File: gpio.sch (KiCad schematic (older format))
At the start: 3 parts, among them J1 DF40C-100DP-0.4V(51), J2 DF40C-100DP-0.4V(51), U1 LFE5U-85F-6BG381C

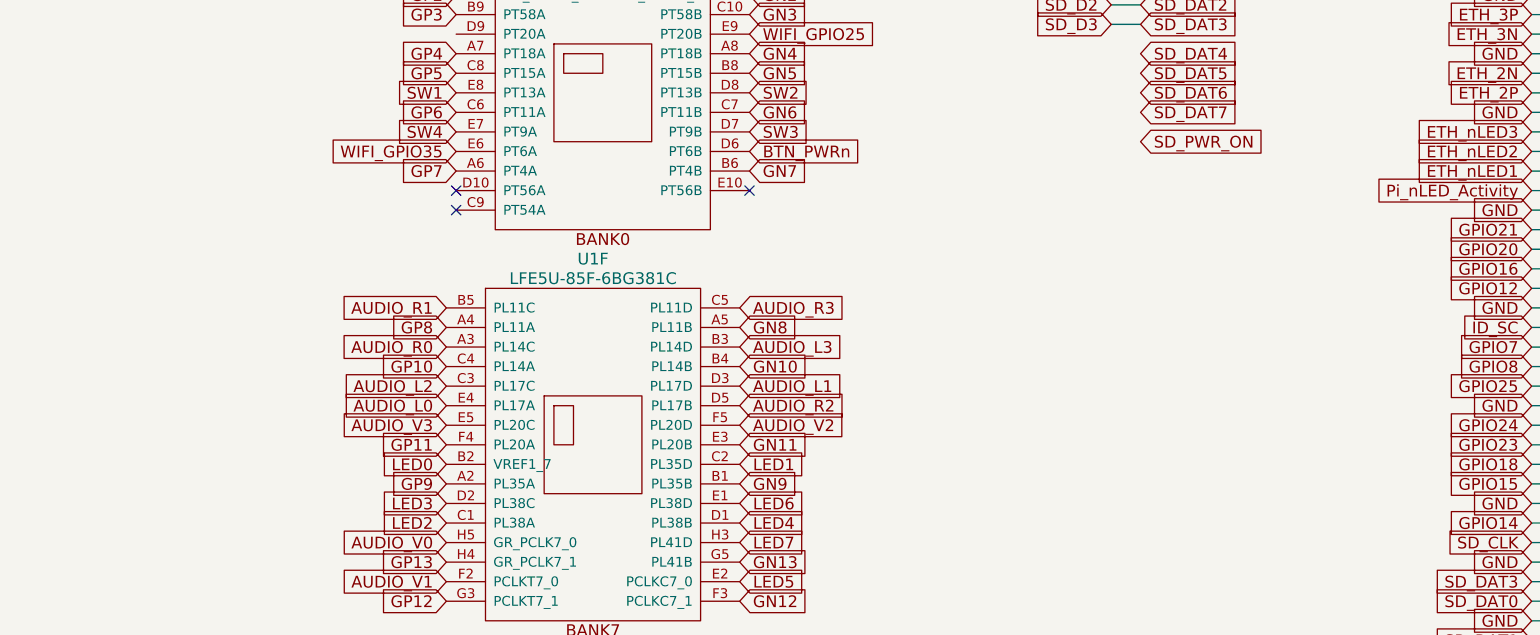
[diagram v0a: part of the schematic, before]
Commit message: SDRAM, JTAG routed - before logo delete
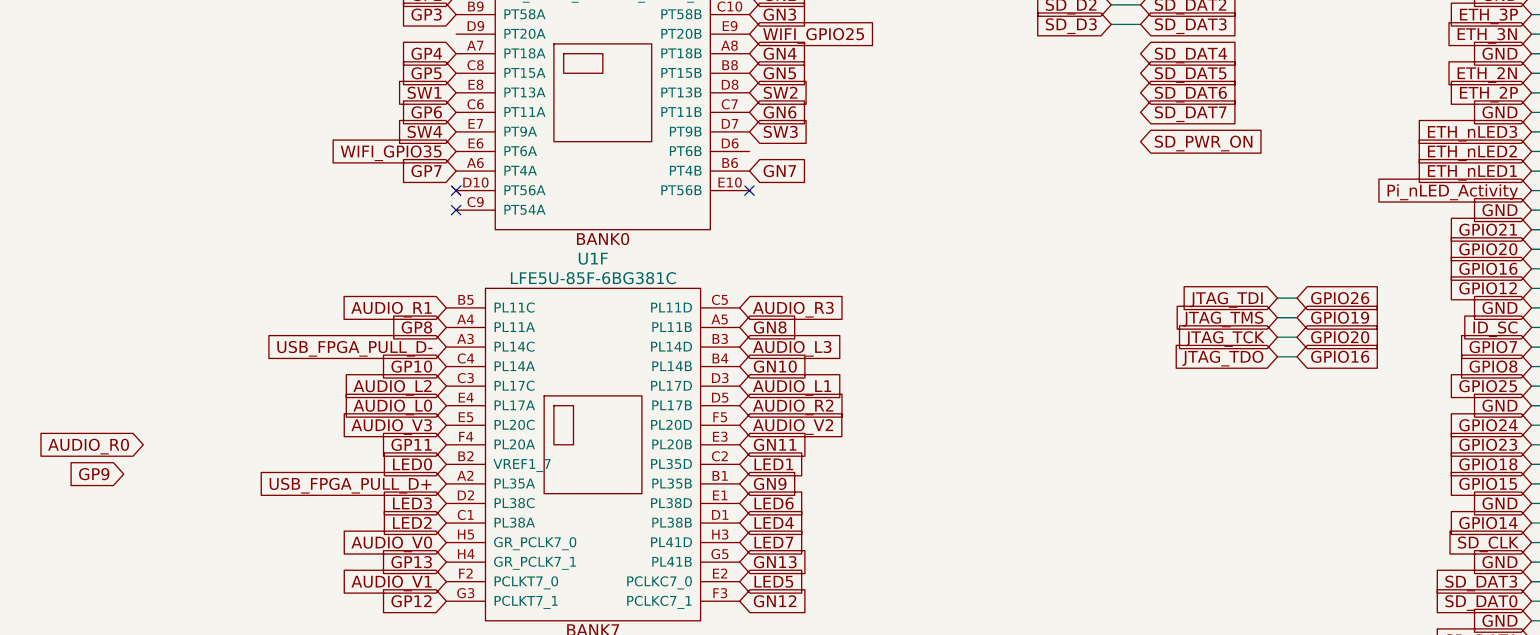
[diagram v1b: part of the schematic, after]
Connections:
- net AUDIO_R0: no longer U1.A3 (PL14C)
- net GP9: no longer U1.A2 (PL35A)
- net BTN_PWRn: no longer names the net of U1.D6 (PT6B)
- new net USB_FPGA_PULL_D+: U1.A2 (PL35A)
- new net USB_FPGA_PULL_D-: U1.A3 (PL14C)
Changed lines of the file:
@@
 Text GLabel 2550 3500 2    60   Input ~ 0
 GN9
-Text GLabel 1050 3500 0    60   Input ~ 0
+Text GLabel -600 3450 0    60   Input ~ 0
 GP9
 Text GLabel 2550 2900 2    60   Input ~ 0
@@
 Text GLabel 2550 2800 2    60   Input ~ 0
 AUDIO_L3
-Text GLabel 1050 2800 0    60   Input ~ 0
+Text GLabel -500 3300 0    60   Input ~ 0
 AUDIO_R0
 Text GLabel 1050 2600 0    60   Input ~ 0
@@
 Text Notes 950  7550 0    60   ~ 0
 GPIO route only A/B pairs as those are differential bidirectional\ndon't route C/D pairs to GPIO as those can be differential input only\nBANK0,1 are single-ended (non-differential)
-Text GLabel 2600 1800 2    60   Input ~ 0
-BTN_PWRn
 Text Notes 950  7200 0    60   ~ 0
 GP,GN 14-21 differential bidirectional connected to BANK2,3 on "ram" sheet\nGP,GN 22-27 single-ended connected to BANK1 on "gpdi" sheet
@@
 Wire Wire Line
 	4600 1150 4450 1150
+Text GLabel 1050 3500 0    60   Input ~ 0
+USB_FPGA_PULL_D+
+Text GLabel 1050 2800 0    60   Input ~ 0
+USB_FPGA_PULL_D-
+Text GLabel 5300 2550 0    60   Input ~ 0
+JTAG_TDI
+Text GLabel 5300 2650 0    60   Input ~ 0
+JTAG_TMS
+Text GLabel 5300 2750 0    60   Input ~ 0
+JTAG_TCK
+Text GLabel 5300 2850 0    60   Input ~ 0
+JTAG_TDO
+Text GLabel 5400 2550 2    60   Input ~ 0
+GPIO26
+Text GLabel 5400 2650 2    60   Input ~ 0
+GPIO19
+Text GLabel 5400 2850 2    60   Input ~ 0
+GPIO16
+Wire Wire Line
+	5300 2550 5400 2550
+Wire Wire Line
+	5400 2650 5300 2650
+Text GLabel 5400 2750 2    60   Input ~ 0
+GPIO20
+Wire Wire Line
+	5300 2750 5400 2750
+Wire Wire Line
+	5400 2850 5300 2850
 $EndSCHEMATC

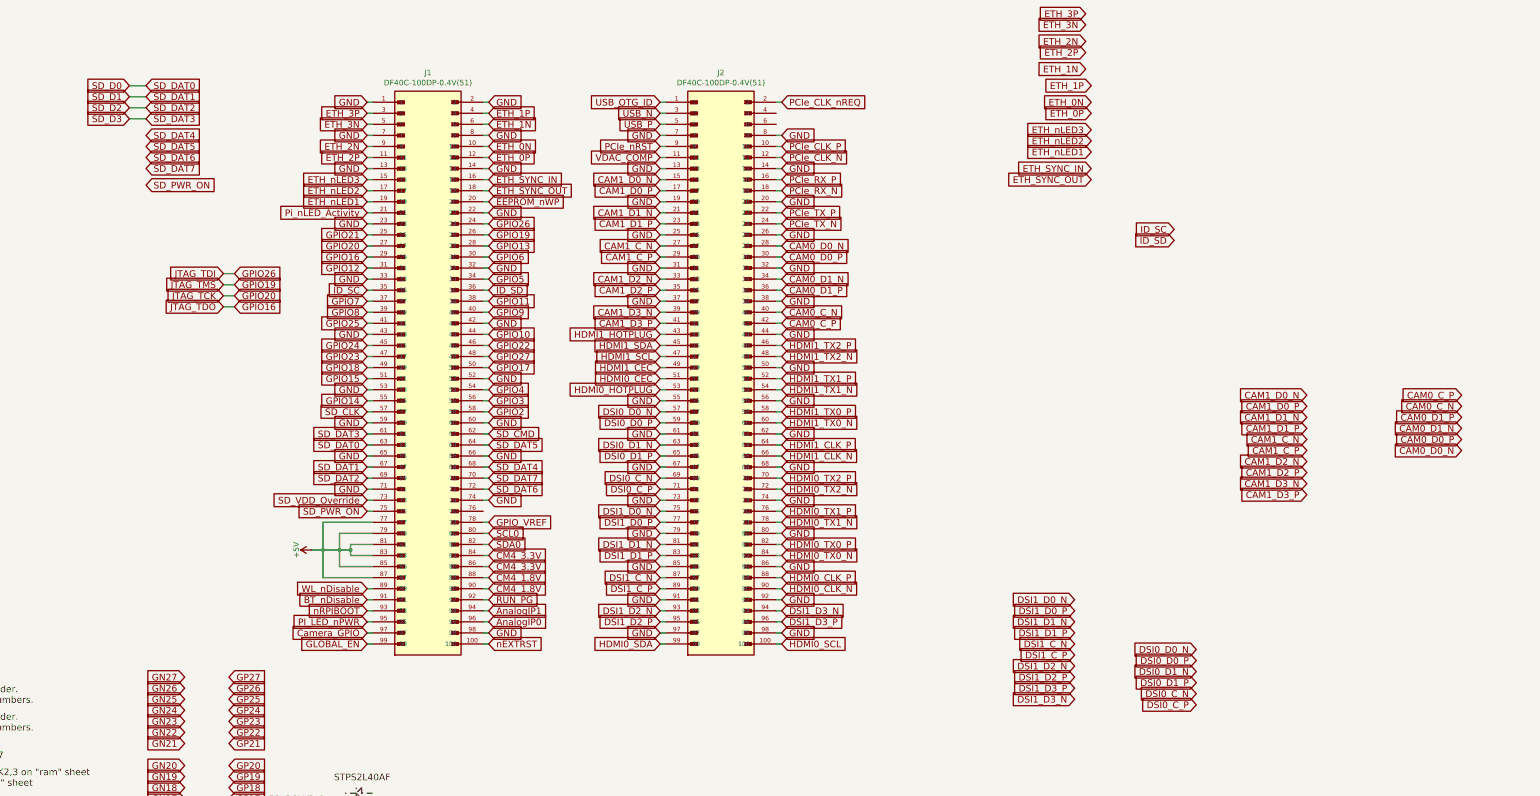
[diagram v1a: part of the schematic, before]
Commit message: Cleaning DRC errors
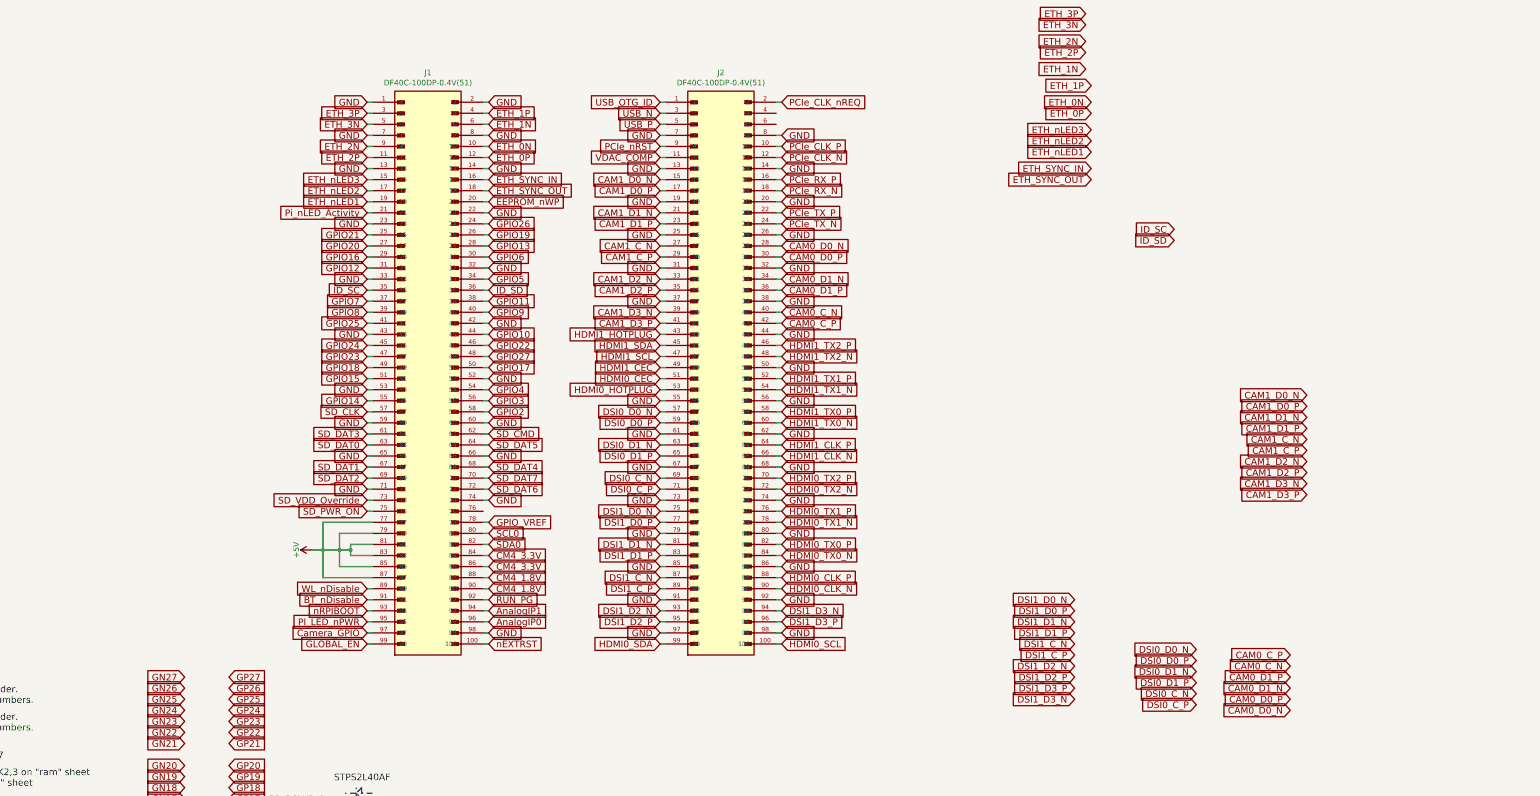
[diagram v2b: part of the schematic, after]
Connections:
- net SD_D0 renamed SD_DAT0
- net SD_D1 renamed SD_DAT1
- net SD_D2 renamed SD_DAT2
- net SD_D3 renamed SD_DAT3
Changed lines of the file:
@@
 Text GLabel 18150 2350 0    60   Input ~ 0
 GPIO21
-Text GLabel 16500 4150 0    60   Input ~ 0
+Text GLabel 14950 6500 0    60   Input ~ 0
 CAM0_D0_N
-Text GLabel 16500 4050 0    60   Input ~ 0
+Text GLabel 14950 6400 0    60   Input ~ 0
 CAM0_D0_P
-Text GLabel 16500 3950 0    60   Input ~ 0
+Text GLabel 14950 6300 0    60   Input ~ 0
 CAM0_D1_N
-Text GLabel 16500 3850 0    60   Input ~ 0
+Text GLabel 14950 6200 0    60   Input ~ 0
 CAM0_D1_P
-Text GLabel 16500 3750 0    60   Input ~ 0
+Text GLabel 14950 6100 0    60   Input ~ 0
 CAM0_C_N
-Text GLabel 16500 3650 0    60   Input ~ 0
+Text GLabel 14950 6000 0    60   Input ~ 0
 CAM0_C_P
 Text GLabel 15100 3650 0    60   Input ~ 0
@@
 Text GLabel 14100 5950 0    60   Input ~ 0
 DSI0_D0_N
-Text GLabel 4450 1050 0    60   Input ~ 0
-SD_D2
-Text GLabel 4450 1150 0    60   Input ~ 0
-SD_D3
-Text GLabel 4450 850  0    60   Input ~ 0
-SD_D0
-Text GLabel 4450 950  0    60   Input ~ 0
-SD_D1
-Text GLabel 4600 1050 2    60   Input ~ 0
-SD_DAT2
-Text GLabel 4600 950  2    60   Input ~ 0
-SD_DAT1
-Text GLabel 4600 1300 2    60   Input ~ 0
-SD_DAT4
-Text GLabel 4600 1400 2    60   Input ~ 0
-SD_DAT5
-Text GLabel 4600 1500 2    60   Input ~ 0
-SD_DAT6
-Text GLabel 4600 1600 2    60   Input ~ 0
-SD_DAT7
-Text GLabel 4600 1150 2    60   Input ~ 0
-SD_DAT3
-Text GLabel 4600 850  2    60   Input ~ 0
-SD_DAT0
-Text GLabel 4600 1750 2    60   Input ~ 0
-SD_PWR_ON
-Wire Wire Line
-	4450 850  4600 850
-Wire Wire Line
-	4600 950  4450 950
-Wire Wire Line
-	4450 1050 4600 1050
-Wire Wire Line
-	4600 1150 4450 1150
 Text GLabel 1050 3500 0    60   Input ~ 0
 USB_FPGA_PULL_D+
 Text GLabel 1050 2800 0    60   Input ~ 0
 USB_FPGA_PULL_D-
-Text GLabel 5300 2550 0    60   Input ~ 0
-JTAG_TDI
-Text GLabel 5300 2650 0    60   Input ~ 0
-JTAG_TMS
-Text GLabel 5300 2750 0    60   Input ~ 0
-JTAG_TCK
-Text GLabel 5300 2850 0    60   Input ~ 0
-JTAG_TDO
-Text GLabel 5400 2550 2    60   Input ~ 0
-GPIO26
-Text GLabel 5400 2650 2    60   Input ~ 0
-GPIO19
-Text GLabel 5400 2850 2    60   Input ~ 0
-GPIO16
-Wire Wire Line
-	5300 2550 5400 2550
-Wire Wire Line
-	5400 2650 5300 2650
-Text GLabel 5400 2750 2    60   Input ~ 0
-GPIO20
-Wire Wire Line
-	5300 2750 5400 2750
-Wire Wire Line
-	5400 2850 5300 2850
 $EndSCHEMATC

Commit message: Routing cam and display differential
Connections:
- net GP2: no longer U1.A9 (GR_PCLK0_1)
- net PCIe_CLK_nREQ: now also U1.A9 (GR_PCLK0_1)
- net PCIe_nRST: now also U1.D9 (PT20A)
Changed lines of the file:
@@
 Text GLabel 1100 900  0    60   Input ~ 0
 GP1
-Text GLabel 1100 1000 0    60   Input ~ 0
+Text GLabel 350  600  0    60   Input ~ 0
 GP2
 Text GLabel 1100 1300 0    60   Input ~ 0
@@
 Text GLabel 18150 2350 0    60   Input ~ 0
 GPIO21
-Text GLabel 14950 6500 0    60   Input ~ 0
-CAM0_D0_N
-Text GLabel 14950 6400 0    60   Input ~ 0
-CAM0_D0_P
-Text GLabel 14950 6300 0    60   Input ~ 0
-CAM0_D1_N
-Text GLabel 14950 6200 0    60   Input ~ 0
-CAM0_D1_P
-Text GLabel 14950 6100 0    60   Input ~ 0
-CAM0_C_N
-Text GLabel 14950 6000 0    60   Input ~ 0
-CAM0_C_P
 Text GLabel 15100 3650 0    60   Input ~ 0
 CAM1_D0_N
@@
 Text GLabel 13000 5500 0    60   Input ~ 0
 DSI1_D0_N
-Text GLabel 14100 6450 0    60   Input ~ 0
-DSI0_C_P
-Text GLabel 14100 6350 0    60   Input ~ 0
-DSI0_C_N
-Text GLabel 14100 6250 0    60   Input ~ 0
-DSI0_D1_P
-Text GLabel 14100 6150 0    60   Input ~ 0
-DSI0_D1_N
-Text GLabel 14100 6050 0    60   Input ~ 0
-DSI0_D0_P
-Text GLabel 14100 5950 0    60   Input ~ 0
-DSI0_D0_N
 Text GLabel 1050 3500 0    60   Input ~ 0
 USB_FPGA_PULL_D+
 Text GLabel 1050 2800 0    60   Input ~ 0
 USB_FPGA_PULL_D-
+Text GLabel 1100 1000 0    60   Input ~ 0
+PCIe_CLK_nREQ
+Text GLabel 1100 1200 0    60   Input ~ 0
+PCIe_nRST
 $EndSCHEMATC
